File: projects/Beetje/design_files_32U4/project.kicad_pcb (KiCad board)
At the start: 2 copper layers, 25.4 x 25.4 mm, 30 parts, among them CON1 AVR-ISP-6, J2 Beetje Bottom, J4 Beetje Top, SW1 RST, SW2 D4, U1 ATMEGA32U4-AU, U2 MIC5225-3.3, X3 USB_OTG, Y1 8 Mhz

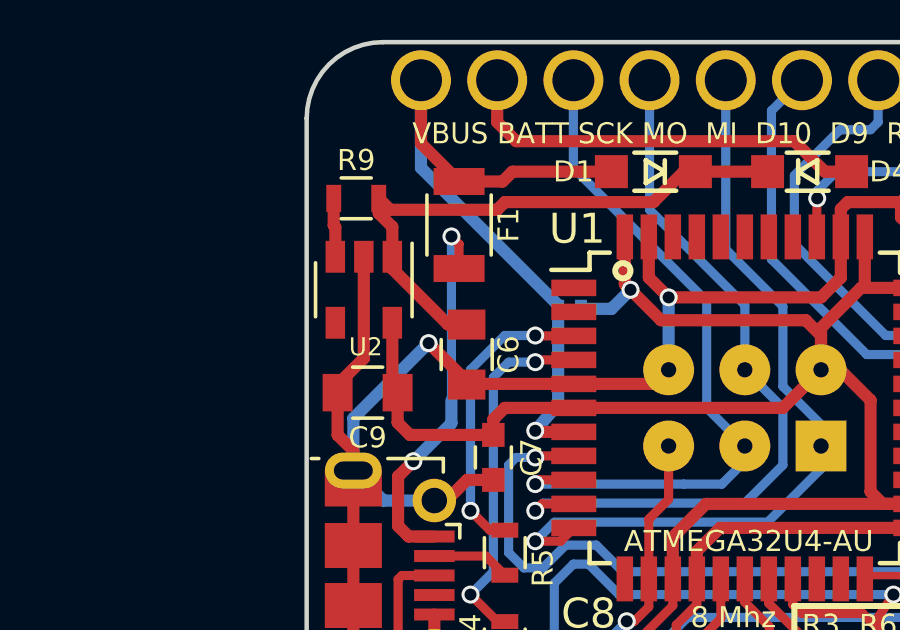
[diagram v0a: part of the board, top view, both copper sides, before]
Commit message: Updates
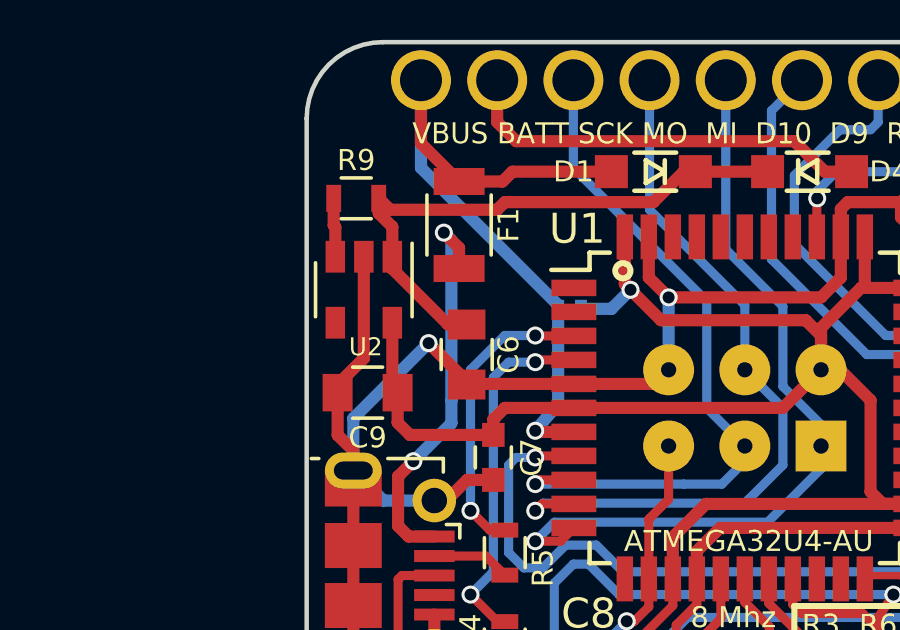
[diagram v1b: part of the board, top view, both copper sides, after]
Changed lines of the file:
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@@
-(kicad_pcb (version 4) (host pcbnew 4.0.6)
+(kicad_pcb (version 4) (host pcbnew 4.0.7)
   (general
     (links 85)
     (no_connects 0)
-    (area 142.164999 86.284999 167.715001 111.835001)
+    (area 125.73 78.580001 182.145715 116.332001)
     (thickness 1.6)
     (drawings 28)
-    (tracks 421)
+    (tracks 422)
     (zones 0)
     (modules 30)
@@
   )
   (setup
-    (last_trace_width 0.3048)
+    (last_trace_width 0.4064)
     (user_trace_width 0.3048)
     (user_trace_width 0.4064)
@@
   (segment (start 164.338 104.013) (end 164.465 104.14) (width 0.3048) (layer B.Cu) (net 36))
   (segment (start 163.576 104.013) (end 164.338 104.013) (width 0.3048) (layer B.Cu) (net 36))
-  (segment (start 165.1 106.172) (end 165.1 106.565) (width 0.3048) (layer F.Cu) (net 36) (status 800000))
+  (segment (start 165.1 106.172) (end 165.1 106.565) (width 0.3048) (layer F.Cu) (net 36))
   (segment (start 164.465 105.537) (end 165.1 106.172) (width 0.3048) (layer F.Cu) (net 36))
   (segment (start 163.195 106.565) (end 162.953 106.565) (width 0.25) (layer F.Cu) (net 37))
@@
   (segment (start 165.443 111.163) (end 167.005 109.601) (width 0.3048) (layer F.Cu) (net 43))
   (segment (start 167.005 109.601) (end 167.005 108.065) (width 0.3048) (layer F.Cu) (net 43))
+  (segment (start 147.066 98.298) (end 147.066 92.964) (width 0.4064) (layer B.Cu) (net 44))
+  (segment (start 145.639 102.84) (end 145.288 102.489) (width 0.4064) (layer F.Cu) (net 44))
+  (segment (start 145.288 102.489) (end 145.288 100.838) (width 0.4064) (layer F.Cu) (net 44))
+  (segment (start 145.288 100.838) (end 145.796 100.33) (width 0.4064) (layer F.Cu) (net 44))
+  (via (at 145.796 100.33) (size 0.6) (drill 0.4) (layers F.Cu B.Cu) (net 44))
+  (segment (start 145.796 100.33) (end 147.066 99.06) (width 0.4064) (layer B.Cu) (net 44))
+  (segment (start 147.066 99.06) (end 147.066 98.298) (width 0.4064) (layer B.Cu) (net 44))
   (segment (start 146.495 102.84) (end 145.639 102.84) (width 0.4064) (layer F.Cu) (net 44))
-  (segment (start 147.066 99.06) (end 147.066 98.298) (width 0.4064) (layer B.Cu) (net 44))
-  (segment (start 145.796 100.33) (end 147.066 99.06) (width 0.4064) (layer B.Cu) (net 44))
-  (via (at 145.796 100.33) (size 0.6) (drill 0.4) (layers F.Cu B.Cu) (net 44))
-  (segment (start 145.288 100.838) (end 145.796 100.33) (width 0.4064) (layer F.Cu) (net 44))
-  (segment (start 145.288 102.489) (end 145.288 100.838) (width 0.4064) (layer F.Cu) (net 44))
-  (segment (start 145.639 102.84) (end 145.288 102.489) (width 0.4064) (layer F.Cu) (net 44))
-  (segment (start 147.32 93.091) (end 147.32 93.906) (width 0.3048) (layer F.Cu) (net 44))
-  (segment (start 147.066 92.837) (end 147.32 93.091) (width 0.3048) (layer F.Cu) (net 44))
-  (via (at 147.066 92.837) (size 0.6) (drill 0.4) (layers F.Cu B.Cu) (net 44))
-  (segment (start 147.066 98.298) (end 147.066 92.837) (width 0.3048) (layer B.Cu) (net 44))
+  (segment (start 147.32 93.218) (end 147.32 93.906) (width 0.4064) (layer F.Cu) (net 44) (status 800000))
+  (segment (start 146.812 92.71) (end 147.32 93.218) (width 0.4064) (layer F.Cu) (net 44))
+  (via (at 146.812 92.71) (size 0.6) (drill 0.4) (layers F.Cu B.Cu) (net 44))
+  (segment (start 147.066 92.964) (end 146.812 92.71) (width 0.4064) (layer B.Cu) (net 44))
   (segment (start 161.29 109.563) (end 161.455 109.563) (width 0.3048) (layer F.Cu) (net 45))
   (segment (start 161.455 109.563) (end 162.953 108.065) (width 0.3048) (layer F.Cu) (net 45))
